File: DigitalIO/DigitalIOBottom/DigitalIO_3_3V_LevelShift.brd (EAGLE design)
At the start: 64 x 82 mm, 76 parts, among them IC1 MCP23017SP, IC2 ULN2803A, K5 HF46105, K6 HF46105, K7 HF46105, K8 HF46105, P1 DF11-06-2DS, Q1 BS170, Q2 BS170, Q5 691131710002, Q6 691131710002, Q7 691131710002, Q8 691131710002, X1 691131710005, X2 691131710004

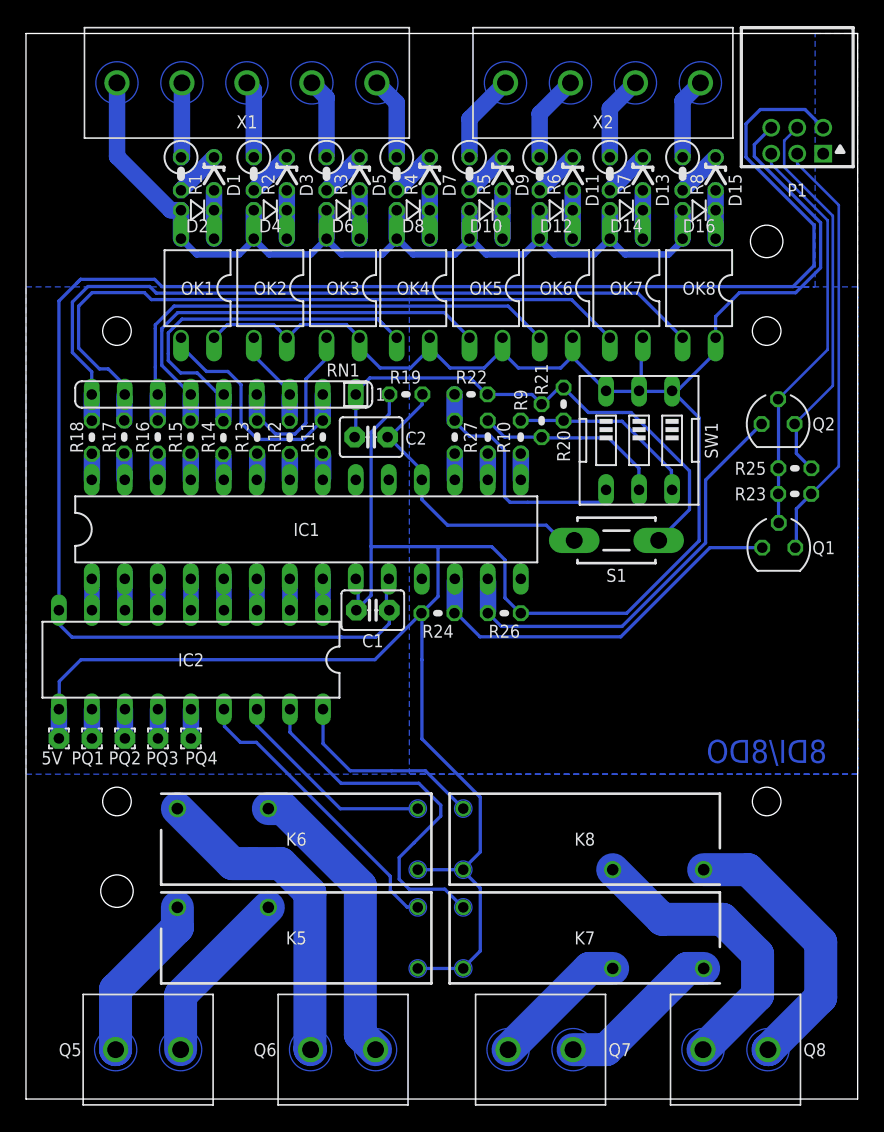
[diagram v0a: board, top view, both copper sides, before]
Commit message: Prepare for production.
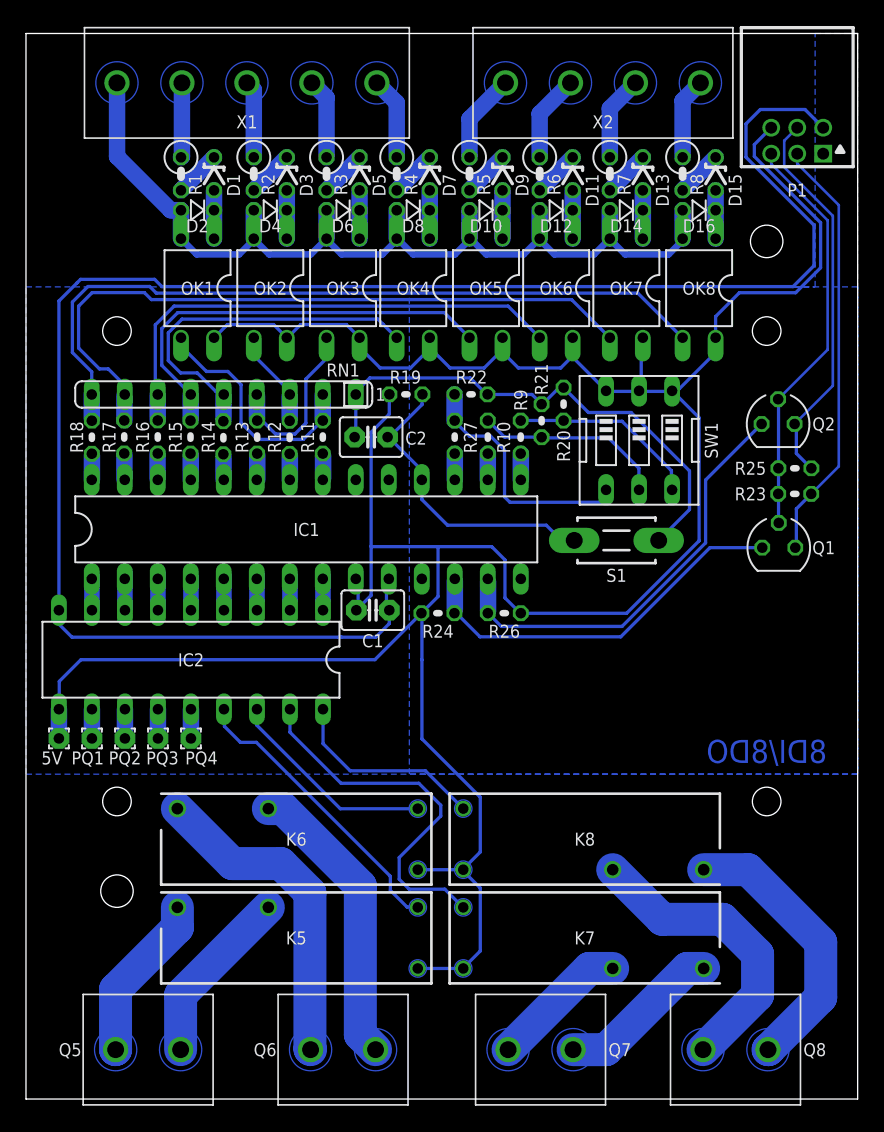
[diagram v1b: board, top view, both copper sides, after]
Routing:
- net N$31: track 29.9 -> 29.3 mm
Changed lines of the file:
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@@
 <wire x1="15.2" y1="54.175" x2="15.22" y2="54.22" width="0.508" layer="16"/>
 <wire x1="28.53" y1="58.57" x2="28.28" y2="58.68" width="0.254" layer="16"/>
-<wire x1="27.08" y1="60.02" x2="27.47" y2="59.63" width="0.254" layer="16"/>
 <wire x1="27.47" y1="59.63" x2="28.53" y2="58.57" width="0.254" layer="16"/>
 <wire x1="13.18" y1="55.88" x2="11.9" y2="55.88" width="0.254" layer="16"/>
@@
 <wire x1="14.62" y1="54.44" x2="15.22" y2="54.22" width="0.254" layer="16"/>
 <wire x1="11.9" y1="55.88" x2="10.95" y2="56.83" width="0.254" layer="16"/>
-<wire x1="10.95" y1="56.83" x2="10.95" y2="57.36" width="0.254" layer="16"/>
-<wire x1="10.95" y1="57.36" x2="10.95" y2="58.96" width="0.254" layer="16"/>
+<wire x1="10.95" y1="56.83" x2="10.95" y2="58.96" width="0.254" layer="16"/>
 <wire x1="10.95" y1="58.96" x2="12.01" y2="60.02" width="0.254" layer="16"/>
 <wire x1="12.01" y1="60.02" x2="27.08" y2="60.02" width="0.254" layer="16"/>
@@
 <wire x1="12.44" y1="54.74" x2="12.17" y2="54.74" width="0.254" layer="16"/>
 <wire x1="12.17" y1="54.74" x2="10.45" y2="56.46" width="0.254" layer="16"/>
-<wire x1="10.45" y1="56.46" x2="10.45" y2="59.13" width="0.254" layer="16"/>
-<wire x1="10.45" y1="59.13" x2="10.45" y2="59.29" width="0.254" layer="16"/>
+<wire x1="10.45" y1="56.46" x2="10.45" y2="59.29" width="0.254" layer="16"/>
 <wire x1="10.45" y1="59.29" x2="11.68" y2="60.52" width="0.254" layer="16"/>
 <wire x1="11.68" y1="60.52" x2="32.2" y2="60.52" width="0.254" layer="16"/>
@@
 <wire x1="10.04" y1="54.74" x2="10.14" y2="54.22" width="0.254" layer="16"/>
 <wire x1="10.04" y1="54.74" x2="9.95" y2="54.83" width="0.254" layer="16"/>
-<wire x1="9.95" y1="54.83" x2="9.95" y2="56.33" width="0.254" layer="16"/>
-<wire x1="9.95" y1="56.33" x2="9.95" y2="59.28" width="0.254" layer="16"/>
-<wire x1="9.95" y1="59.28" x2="9.95" y2="59.57" width="0.254" layer="16"/>
+<wire x1="9.95" y1="54.83" x2="9.95" y2="59.57" width="0.254" layer="16"/>
 <wire x1="9.95" y1="59.57" x2="11.4" y2="61.02" width="0.254" layer="16"/>
 <wire x1="11.4" y1="61.02" x2="37.1" y2="61.02" width="0.254" layer="16"/>
@@
 </polygon>
 <wire x1="31.92" y1="22.61" x2="31.92" y2="21.78" width="0.254" layer="16"/>
-<wire x1="31.92" y1="21.78" x2="29.86" y2="19.72" width="0.254" layer="16"/>
-<wire x1="29.86" y1="19.72" x2="28.72" y2="18.58" width="0.254" layer="16"/>
+<wire x1="31.92" y1="21.78" x2="28.72" y2="18.58" width="0.254" layer="16"/>
 <wire x1="28.72" y1="18.58" x2="28.72" y2="16.92" width="0.254" layer="16"/>
 <wire x1="28.72" y1="16.92" x2="29.49" y2="16.15" width="0.254" layer="16"/>
@@
 </polygon>
 <wire x1="33.65" y1="22.35" x2="30.74" y2="25.26" width="0.254" layer="16"/>
-<wire x1="30.74" y1="25.26" x2="28.11" y2="25.26" width="0.254" layer="16"/>
-<wire x1="28.11" y1="25.26" x2="24.95" y2="25.26" width="0.254" layer="16"/>
+<wire x1="30.74" y1="25.26" x2="24.95" y2="25.26" width="0.254" layer="16"/>
 <wire x1="24.95" y1="25.26" x2="22.86" y2="27.35" width="0.254" layer="16"/>
 <wire x1="22.86" y1="27.35" x2="22.86" y2="29.994884375" width="0.254" layer="16"/>
@@
 </polygon>
 <wire x1="11.65" y1="22.35" x2="15.88" y2="18.12" width="2.54" layer="16"/>
-<wire x1="15.88" y1="18.12" x2="17.48" y2="18.12" width="2.54" layer="16"/>
-<wire x1="17.48" y1="18.12" x2="19.61" y2="18.12" width="2.54" layer="16"/>
+<wire x1="15.88" y1="18.12" x2="19.61" y2="18.12" width="2.54" layer="16"/>
 <wire x1="19.61" y1="18.12" x2="21.85" y2="15.88" width="2.54" layer="16"/>
 <wire x1="21.85" y1="15.88" x2="21.85" y2="3.85" width="2.54" layer="16"/>
@@
 <contactref element="K8" pad="NO"/>
 <contactref element="Q8" pad="1"/>
-<wire x1="61.12" y1="7.79" x2="57.13" y2="3.8" width="2.54" layer="16"/>
+<wire x1="61.16" y1="7.83" x2="57.13" y2="3.8" width="2.54" layer="16"/>
 <wire x1="57.13" y1="3.8" x2="57.1" y2="3.8" width="2.54" layer="16"/>
 <polygon width="0.35" layer="16" thermals="no">
@@
 <wire x1="55.57" y1="17.65" x2="61.16" y2="12.06" width="2.54" layer="16"/>
 <wire x1="61.16" y1="12.06" x2="61.16" y2="7.83" width="2.54" layer="16"/>
-<wire x1="61.16" y1="7.83" x2="61.12" y2="7.79" width="2.54" layer="16"/>
 </signal>
 <signal name="N$40">
@@
 <wire x1="41.36" y1="54.74" x2="41.37" y2="54.75" width="0.254" layer="16"/>
 <wire x1="39.8" y1="53.52" x2="39.68" y2="53.47" width="0.254" layer="16"/>
-<wire x1="43.2816" y1="52.832" x2="45.9232" y2="52.832" width="0.254" layer="16"/>
+<wire x1="43.2816" y1="52.832" x2="46.568" y2="52.832" width="0.254" layer="16"/>
 <wire x1="41.4528" y1="54.6608" x2="43.2816" y2="52.832" width="0.254" layer="16"/>
 <wire x1="41.4528" y1="54.6608" x2="41.37" y2="54.75" width="0.254" layer="16"/>
@@
 <wire x1="61.35" y1="74.75" x2="59.95" y2="76.15" width="0.254" layer="16"/>
 <wire x1="59.95" y1="76.15" x2="56.51" y2="76.15" width="0.254" layer="16"/>
-<wire x1="4.2" y1="63.08" x2="3.935" y2="62.815" width="0.254" layer="16"/>
 <wire x1="3.935" y1="62.815" x2="2.534884375" y2="61.414884375" width="0.254" layer="16"/>
 <wire x1="2.534884375" y1="61.414884375" x2="2.534884375" y2="37.62" width="0.254" layer="16"/>
-<wire x1="51.5" y1="62.52" x2="10.46" y2="62.52" width="0.254" layer="16"/>
+<wire x1="59.03" y1="62.52" x2="10.46" y2="62.52" width="0.254" layer="16"/>
 <wire x1="10.46" y1="62.52" x2="9.9" y2="63.08" width="0.254" layer="16"/>
 <wire x1="9.9" y1="63.08" x2="4.2" y2="63.08" width="0.254" layer="16"/>
@@
 <wire x1="60.64" y1="67.25" x2="60.64" y2="64.13" width="0.254" layer="16"/>
 <wire x1="60.64" y1="64.13" x2="59.03" y2="62.52" width="0.254" layer="16"/>
-<wire x1="59.03" y1="62.52" x2="51.5" y2="62.52" width="0.254" layer="16"/>
-<wire x1="45.9232" y1="52.832" x2="46.568" y2="52.832" width="0.254" layer="16"/>
 <wire x1="46.568" y1="52.832" x2="51.06" y2="48.34" width="0.254" layer="16"/>
 <wire x1="51.06" y1="48.34" x2="51.06" y2="45.36" width="0.254" layer="16"/>
@@
 <wire x1="61.15" y1="67.44" x2="61.15" y2="63.97" width="0.254" layer="16"/>
 <wire x1="53.09" y1="58.61" x2="53.07" y2="58.59" width="0.254" layer="16"/>
-<wire x1="49.73" y1="54.5" x2="49.72" y2="54.5" width="0.254" layer="16"/>
 <wire x1="38.14" y1="37.35" x2="38.17" y2="37.38" width="0.254" layer="16"/>
 <wire x1="38.17" y1="37.38" x2="46.22" y2="37.38" width="0.254" layer="16"/>
@@
 <wire x1="38.08" y1="52.22" x2="38.07" y2="52.21" width="0.254" layer="16"/>
 <wire x1="41.36" y1="52.22" x2="41.37" y2="52.21" width="0.254" layer="16"/>
-<wire x1="41.48" y1="52.16" x2="43.98" y2="52.16" width="0.254" layer="16"/>
+<wire x1="41.48" y1="52.16" x2="45.87" y2="52.16" width="0.254" layer="16"/>
 <wire x1="41.48" y1="52.16" x2="41.37" y2="52.21" width="0.254" layer="16"/>
-<wire x1="43.98" y1="52.16" x2="45.87" y2="52.16" width="0.254" layer="16"/>
 <wire x1="45.87" y1="52.16" x2="49.67" y2="48.36" width="0.254" layer="16"/>
 <wire x1="49.67" y1="48.36" x2="49.67" y2="46.93" width="0.254" layer="16"/>
@@
 <wire x1="35.54" y1="52.2" x2="35.54" y2="52.21" width="0.254" layer="16"/>
 <wire x1="39.68" y1="50.94" x2="39.68" y2="50.93" width="0.254" layer="16"/>
-<wire x1="39.8" y1="50.88" x2="42.72" y2="50.88" width="0.254" layer="16"/>
+<wire x1="39.8" y1="50.88" x2="44.83" y2="50.88" width="0.254" layer="16"/>
 <wire x1="39.8" y1="50.88" x2="39.68" y2="50.93" width="0.254" layer="16"/>
-<wire x1="42.72" y1="50.88" x2="44.83" y2="50.88" width="0.254" layer="16"/>
 <wire x1="44.83" y1="50.88" x2="47.17" y2="48.54" width="0.254" layer="16"/>
 <wire x1="47.17" y1="48.54" x2="47.17" y2="46.89" width="0.254" layer="16"/>
@@
 <wire x1="32.98" y1="54.23" x2="32.98" y2="52.22" width="1.27" layer="16"/>
 <wire x1="32.98" y1="52.22" x2="32.99" y2="52.21" width="0.254" layer="16"/>
-<wire x1="37.242" y1="45.9232" x2="38.608" y2="45.9232" width="0.254" layer="16"/>
 <wire x1="36.826" y1="46.3392" x2="37.242" y2="45.9232" width="0.254" layer="16"/>
 <wire x1="36.826" y1="49.9404" x2="36.826" y2="46.3392" width="0.254" layer="16"/>
@@
 <wire x1="33.1216" y1="52.0192" x2="34.1244" y2="51.0164" width="0.254" layer="16"/>
 <wire x1="33.1216" y1="52.0192" x2="32.99" y2="52.21" width="0.254" layer="16"/>
-<wire x1="38.608" y1="45.9232" x2="44.2532" y2="45.9232" width="0.254" layer="16"/>
+<wire x1="37.242" y1="45.9232" x2="44.2532" y2="45.9232" width="0.254" layer="16"/>
 <wire x1="44.2532" y1="45.9232" x2="44.64" y2="46.31" width="0.254" layer="16"/>
 <wire x1="44.64" y1="46.31" x2="44.64" y2="46.88" width="0.254" layer="16"/>
